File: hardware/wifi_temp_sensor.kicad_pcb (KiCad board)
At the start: 2 copper layers, 50 x 77 mm, 47 parts, among them IC2 BQ21040DBVR, J2 Batt_Conn, J3 Conn_02x03_Odd_Even, P1 USB_C_Plug_USB2.0, Q1 SSM6L09FUTE85LF, Q2 AO3401A, Q3 BSS214NW, SW1 SW_SPST, SW2 SW_Push, U1 ESP32-C3-WROOM-02, U2 SHT4x, U3 WE-TVS-82400102, U4 LD1117S33TR_SOT223

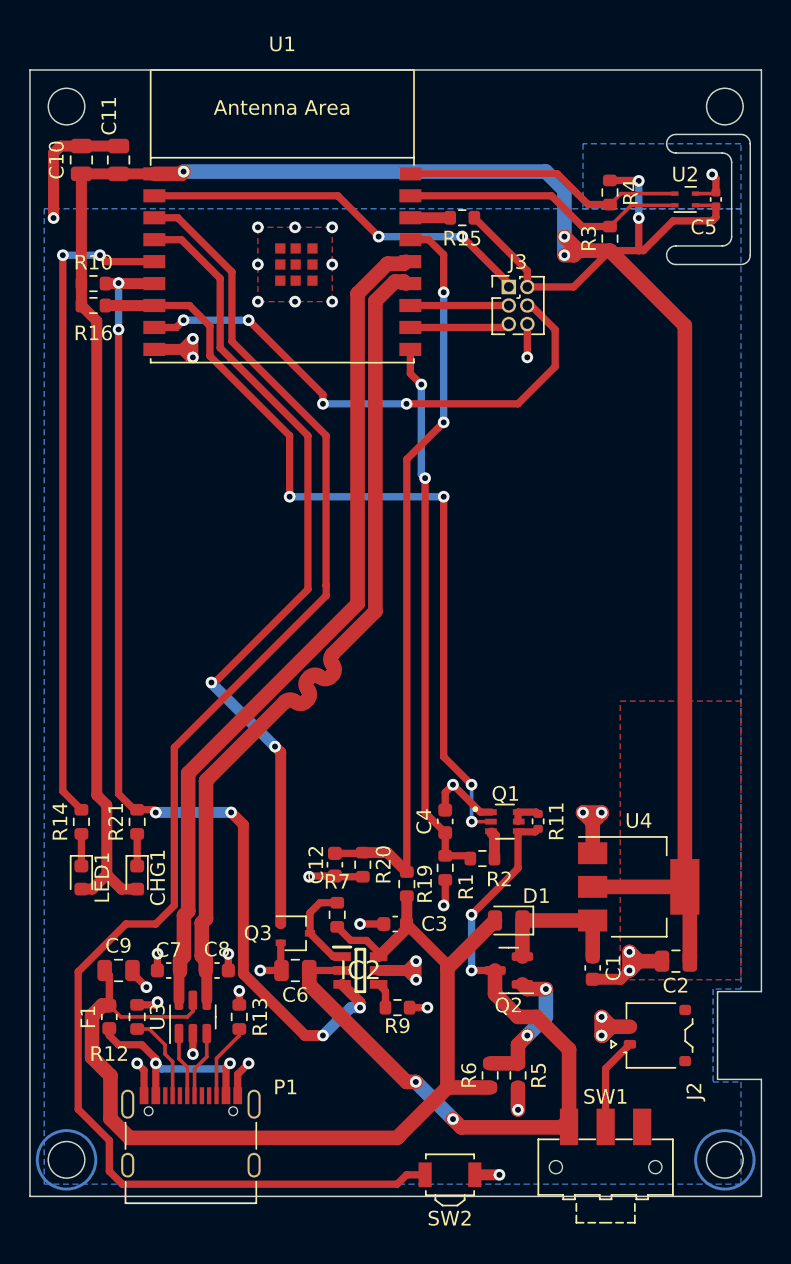
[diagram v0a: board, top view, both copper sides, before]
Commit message: minor changes
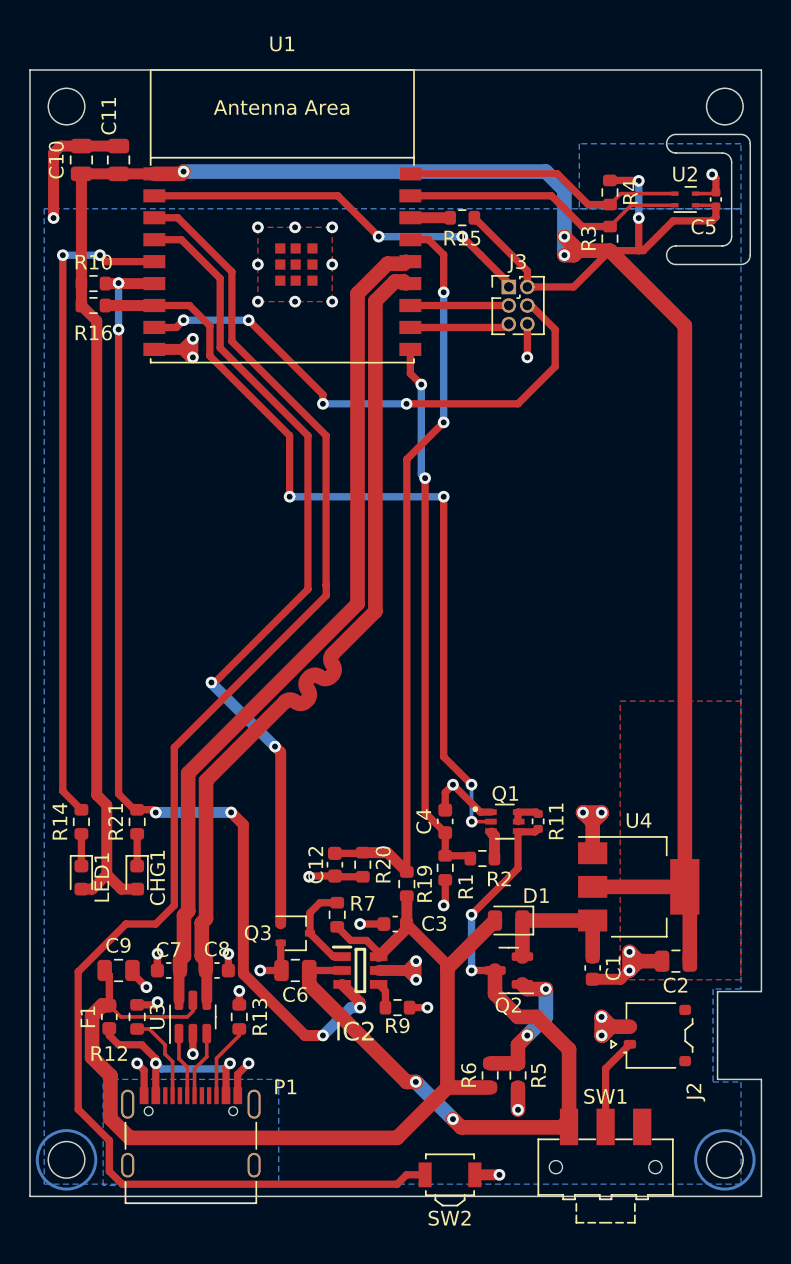
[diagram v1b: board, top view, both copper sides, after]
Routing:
- added copper zone on B.Cu, net unconnected-(P1-SHIELD-PadS1)
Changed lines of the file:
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@@
     (property "ki_description" "0.8A Single Input Single-Cell Li-Ion and Li-Pol Battery Charger")
     (attr smd)
-    (fp_text reference "IC2" (at 0 0) (layer "F.SilkS")
+    (fp_text reference "IC2" (at -0.335 4.195 180) (layer "F.SilkS")
         (effects (font (size 1.27 1.27) (thickness 0.254)))
     )
@@
     (property "ki_keywords" "R resistor")
     (attr smd)
-    (fp_text reference "R7" (at 2.25 0) (layer "F.SilkS")
+    (fp_text reference "R7" (at 0.75 1.75) (layer "F.SilkS")
         (effects (font (size 1 1) (thickness 0.15)))
     )
@@
         (xy 228.6 38.735)
         (xy 228.6 34.29)
-        (xy 217.805 34.29)
-        (xy 217.805 38.735)
+        (xy 217.555 34.29)
+        (xy 217.555 38.735)
       )
     )
@@
       )
     )
+  )
+  (zone (net 22) (net_name "unconnected-(P1-SHIELD-PadS1)") (layer "B.Cu") (hatch edge 0.5)
+    (priority 4)
+    (connect_pads (clearance 0.5))
+    (min_thickness 0.25) (filled_areas_thickness no)
+    (fill yes (thermal_gap 0.5) (thermal_bridge_width 0.5))
+    (polygon
+      (pts
+        (xy 185 98.25)
+        (xy 197 98.25)
+        (xy 197 105.5)
+        (xy 185 105.5)
+      )
+    )
